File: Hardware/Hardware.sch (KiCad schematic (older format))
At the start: 17 parts, among them J1 Conn_01x02, J2 Conn_01x04, J4 Conn_01x02, J6 Conn_01x08, J7 Conn_01x03, U1 ESP32-WROOM-32

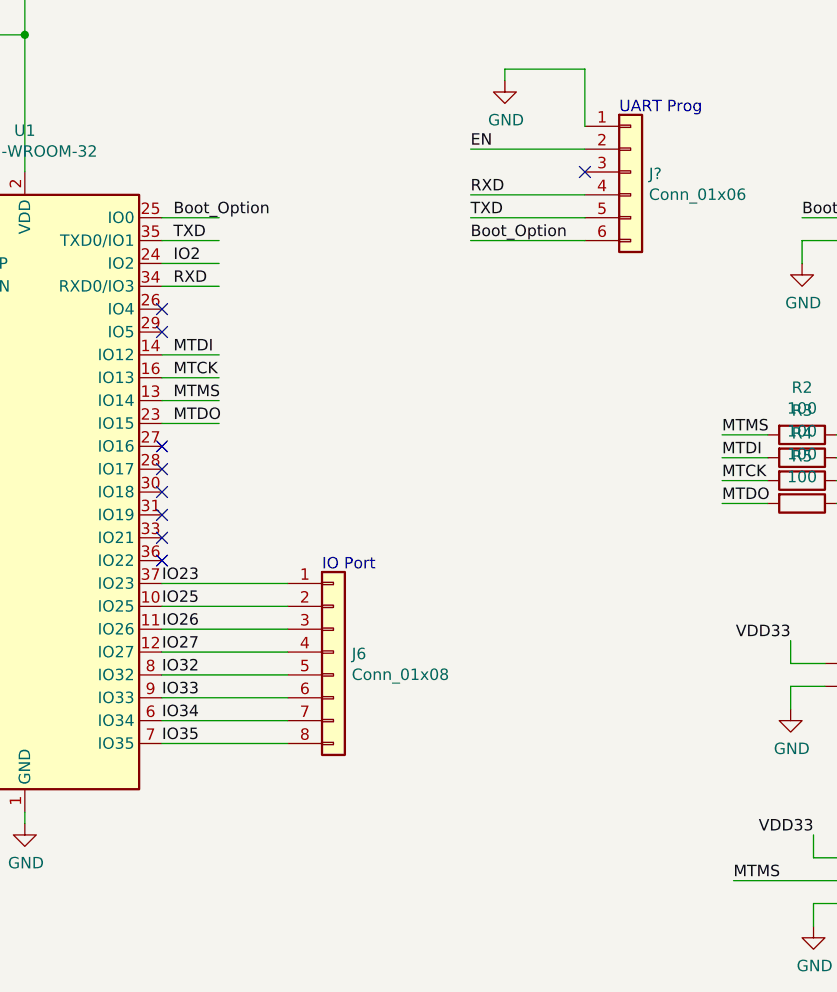
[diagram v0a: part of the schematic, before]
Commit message: layout reworking
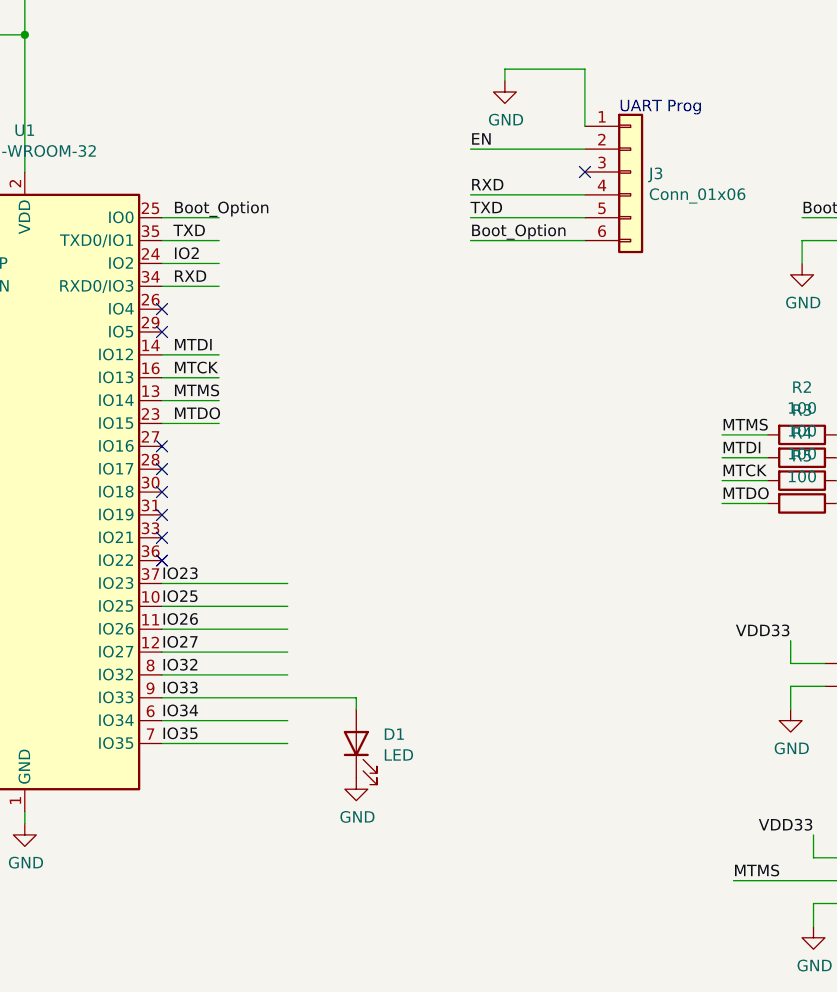
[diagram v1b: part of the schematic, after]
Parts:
- removed J6: Conn_01x08, Connector_PinHeader_2.54mm:PinHeader_1x08_P2.54mm_Vertical, symbol Connector_Generic:Conn_01x08
- added D1: LED, LED_SMD:LED_0805_2012Metric_Castellated, symbol Device:LED
- J3: renamed from J?; footprint (none) -> Connector_PinHeader_2.54mm:PinHeader_1x06_P2.54mm_Vertical
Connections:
- wire segments 59 -> 60
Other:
- note removed: "IO Port"
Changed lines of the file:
@@
 Text Notes 6250 4400 0    50   ~ 0
 Battery Input
-$Comp
-L Connector_Generic:Conn_01x08 J6
-U 1 1 620BF760
-P 3950 4400
-F 0 "J6" H 4030 4392 50  0000 L CNN
-F 1 "Conn_01x08" H 4030 4301 50  0000 L CNN
-F 2 "Connector_PinHeader_2.54mm:PinHeader_1x08_P2.54mm_Vertical" H 3950 4400 50  0001 C CNN
-F 3 "~" H 3950 4400 50  0001 C CNN
-	1    3950 4400
-	1    0    0    -1
-$EndComp
-Wire Wire Line
-	3200 4800 3750 4800
-Wire Wire Line
-	3750 4700 3200 4700
-Wire Wire Line
-	3200 4600 3750 4600
-Wire Wire Line
-	3200 4500 3750 4500
-Wire Wire Line
-	3200 4400 3750 4400
-Wire Wire Line
-	3750 4300 3200 4300
-Wire Wire Line
-	3200 4200 3750 4200
-Wire Wire Line
-	3750 4100 3200 4100
-Text Notes 3900 4050 0    50   ~ 0
-IO Port
 Text Label 3200 4100 0    50   ~ 0
 IO23
@@
 $EndComp
 $Comp
-L Connector_Generic:Conn_01x06 J?
+L Connector_Generic:Conn_01x06 J3
 U 1 1 625FEE76
 P 5250 2300
-F 0 "J?" H 5330 2292 50  0000 L CNN
+F 0 "J3" H 5330 2292 50  0000 L CNN
 F 1 "Conn_01x06" H 5330 2201 50  0000 L CNN
-F 2 "" H 5250 2300 50  0001 C CNN
+F 2 "Connector_PinHeader_2.54mm:PinHeader_1x06_P2.54mm_Vertical" H 5250 2300 50  0001 C CNN
 F 3 "~" H 5250 2300 50  0001 C CNN
 	1    5250 2300
@@
 Text Label 4550 2500 0    50   ~ 0
 TXD
+Wire Wire Line
+	3750 4100 3200 4100
+Wire Wire Line
+	3200 4200 3750 4200
+Wire Wire Line
+	3750 4300 3200 4300
+Wire Wire Line
+	3200 4400 3750 4400
+Wire Wire Line
+	3200 4500 3750 4500
+Wire Wire Line
+	3750 4700 3200 4700
+Wire Wire Line
+	3200 4800 3750 4800
+$Comp
+L Device:LED D1
+U 1 1 6263E05E
+P 4050 4800
+F 0 "D1" V 4089 4682 50  0000 R CNN
+F 1 "LED" V 3998 4682 50  0000 R CNN
+F 2 "LED_SMD:LED_0805_2012Metric_Castellated" H 4050 4800 50  0001 C CNN
+F 3 "~" H 4050 4800 50  0001 C CNN
+	1    4050 4800
+	0    -1   -1   0
+$EndComp
+Wire Wire Line
+	4050 4600 4050 4650
+Wire Wire Line
+	3200 4600 4050 4600
+$Comp
+L power:GND #PWR0110
+U 1 1 62640CA7
+P 4050 4950
+F 0 "#PWR0110" H 4050 4700 50  0001 C CNN
+F 1 "GND" H 4055 4777 50  0000 C CNN
+F 2 "" H 4050 4950 50  0001 C CNN
+F 3 "" H 4050 4950 50  0001 C CNN
+	1    4050 4950
+	1    0    0    -1
+$EndComp
 $EndSCHEMATC
